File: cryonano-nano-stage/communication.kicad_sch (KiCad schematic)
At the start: 47 parts, among them IC1 KSZ8081MLXCA-TR, J6 RJ45_Hanrun_HR911105A_Horizon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, J7 10118194-0001LF, J9 USB4930-00-A, U10 LAN8742A, U2 SRDA3.3-4BTG, U5 ECMF02-2AMX6, Y3 25.0MHz

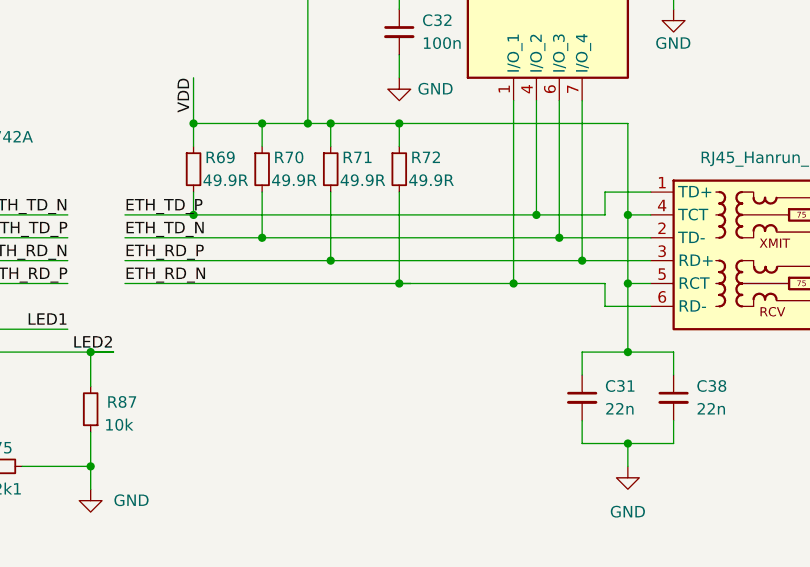
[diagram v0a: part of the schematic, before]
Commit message: drc ok, review schematic
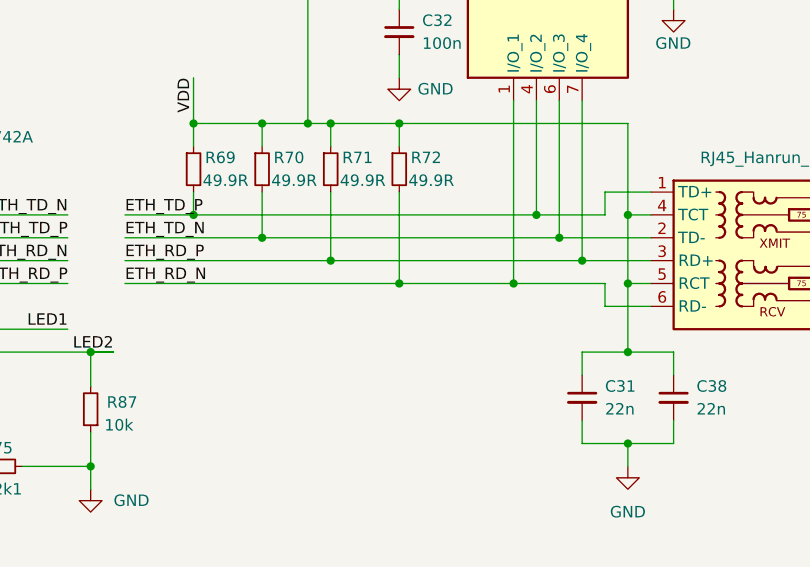
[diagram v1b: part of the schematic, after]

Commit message: release candidate
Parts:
- IC1: Order No. (none) -> KSZ8081MLXCA-TR
- R57, R58, R59, R60, R61, R62, R63, R64, R65, R66, R67, R69, R70, R71, R72, R73, R74, R75, R76, R87, R90: Order No. 0603/120mW -> 0603, 120mW
